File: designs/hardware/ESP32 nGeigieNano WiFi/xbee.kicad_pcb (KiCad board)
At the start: 2 copper layers, 25.5 x 33.2 mm, 6 parts, among them SW1 TACT-SWITCH, SW2 SWITCH_INV, U1 ESP32S

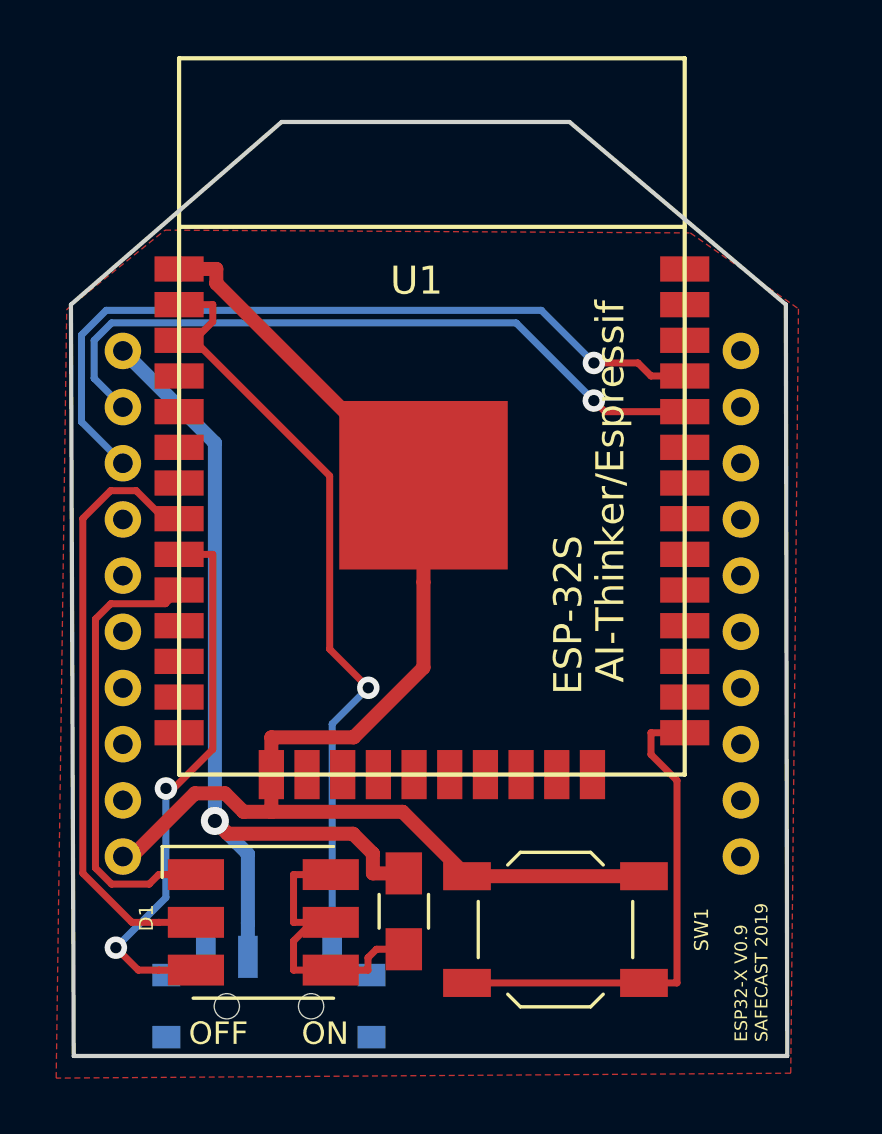
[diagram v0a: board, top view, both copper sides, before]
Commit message: updated files
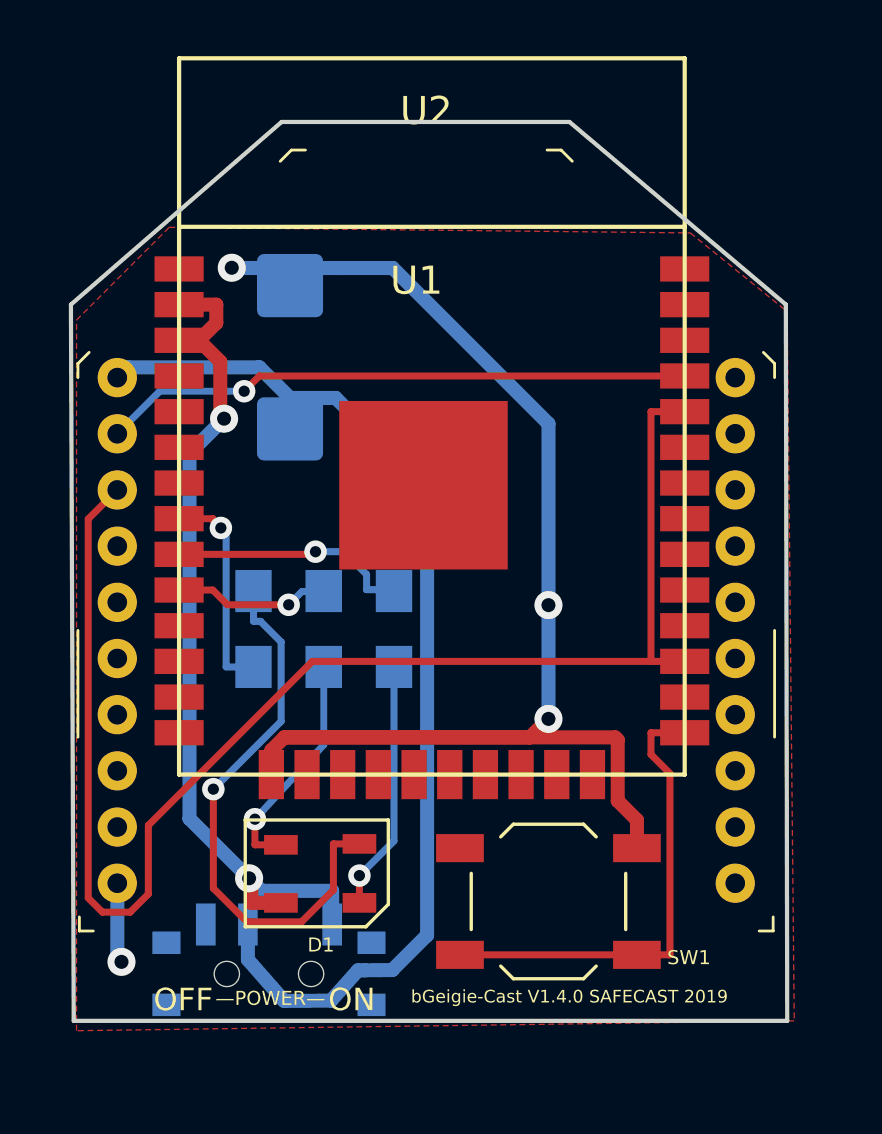
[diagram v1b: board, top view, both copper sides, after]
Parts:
- removed U$1: XBEE-1B2, digikey-footprints:XBEE-20_THT
- added C1: CP1, Capacitor_Tantalum_SMD:CP_EIA-6032-15_Kemet-U_Pad2.25x2.35mm_HandSolder, B.Cu at (143.6, 98.6)
- added G***: LOGO, ESP32 nGeigieNano WiFi all:QR_code_safecast_bgc, B.Cu at (153.1, 116.5)
- added R3: 470, Resistors_SMD:R_0805_HandSoldering, B.Cu at (142.2, 108.3)
- added R4: 470, Resistors_SMD:R_0805_HandSoldering, B.Cu at (147.2, 108.3)
- added U2: XBEE-socket, digikey-footprints:XBEE-20_THT, F.Cu at (148.4, 108.3)
- D1: footprint LEDs:LED_RGB_5050-6 -> digikey-footprints:DJS-BRGBC-TR8
- R1: moved to B.Cu
- moved R1 10.4 mm to (144.8, 108.3), turned to -90 degrees
- moved D1 2.77 mm to (144.8, 117.0), turned to 90 degrees
- moved SW2 1.15 mm to (142.8, 120.2)
- moved SW1 1.03 mm to (152.8, 118.0)
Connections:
- D1 pad 2: Net-(D1-Pad2) -> +3V3
- R1 pad 1: Net-(D1-Pad4) -> Net-(R1-Pad1)
- R1 pad 2: VDD -> Net-(D1-Pad3)
- SW2 pad 1: Net-(SW2-Pad1) -> +3V3
- U1 pad 10: Net-(D1-Pad1) -> Net-(R1-Pad1)
- U1 pad 2: Net-(SW2-Pad1) -> +3V3
- U1 pad 27: (no net) -> Net-(U1-Pad27)
- U1 pad 3: Net-(SW2-Pad1) -> +3V3
- U1 pad 34: Net-(U$1-Pad2) -> Net-(U1-Pad27)
- U1 pad 8: Net-(D1-Pad2) -> Net-(R3-Pad1)
- U1 pad 9: Net-(D1-Pad3) -> Net-(R4-Pad1)
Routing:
- net Net-(U1-Pad27): track 0.00 -> 51.6 mm
- net +3V3: track 0.00 -> 30.8 mm, vias 0 -> 2
- net Net-(SW2-Pad1): track 28.3 -> 0.00 mm, vias 1 -> 0
- net Net-(U$1-Pad2): track 25.4 -> 0.00 mm, vias 1 -> 0
- net Net-(D1-Pad2): track 21.6 -> 0.00 mm
- net Net-(D1-Pad3): track 20.0 -> 8.22 mm, vias 2 -> 1
- net Net-(D1-Pad4): track 10.8 -> 19.9 mm, vias 0 -> 1
- net Net-(R4-Pad1): track 0.00 -> 8.57 mm, vias 0 -> 1
- net VDD: track 31.3 -> 39.9 mm, vias 1 -> 0
- net Net-(R3-Pad1): track 0.00 -> 7.65 mm, vias 0 -> 1
- net Net-(D1-Pad1): track 16.2 -> 8.96 mm, vias 0 -> 1
- net Net-(U1-Pad35): track 28.0 -> 21.1 mm
- net GND: track 48.6 -> 54.2 mm, vias 0 -> 4
- net Net-(R1-Pad1): track 0.00 -> 5.57 mm, vias 0 -> 1
- net Net-(SW1-Pad1): track 18.0 -> 16.9 mm
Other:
- board size 25.5 x 33.2 mm -> 25.5 x 32 mm
- net class Default removed
- net class Power removed
- board text added: "Scan QR code for manual bGeigie-Cast V1.4.0 info@safecast.org"
- board text added: "bGeigie-Cast V1.4.0 SAFECAST 2019"
- board text added: "https://safecast.org/bgc"
- board text added: "—POWER—"
- board text removed: "ESP32-X V0.9 SAFECAST 2019"
